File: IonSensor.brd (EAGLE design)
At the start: 50.8 x 22.9 mm, 44 parts, among them IC1 QUAD_OPAMPD, IC2 QUAD_OPAMPD, IC3 QUAD_OPAMPD, X1 B5B-XH-2

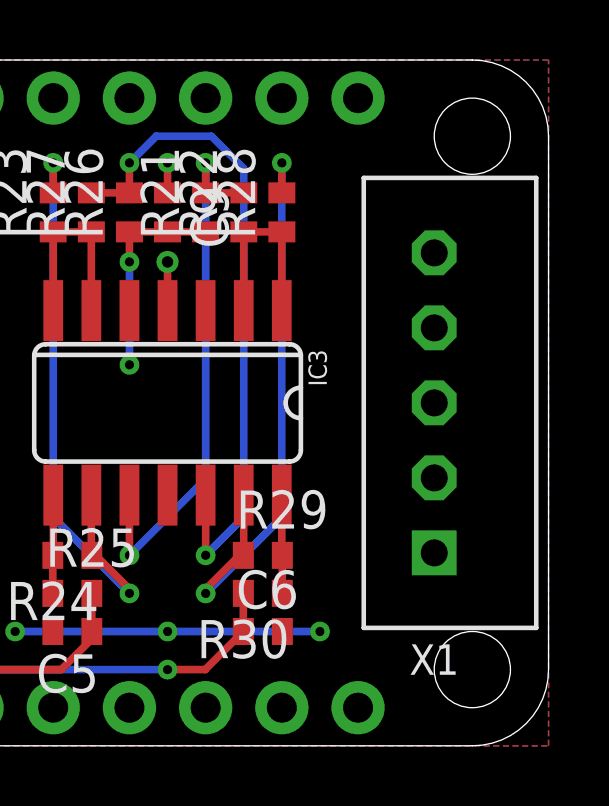
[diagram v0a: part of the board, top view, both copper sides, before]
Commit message: Revert "Added JST XH Connector"
This reverts commit 28e9dc296f10d82968848f6f33b36970200c6171.
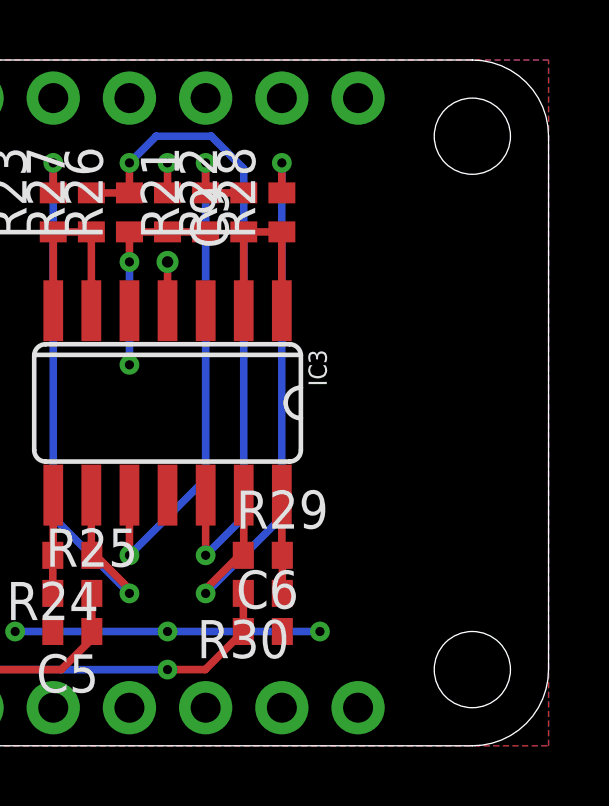
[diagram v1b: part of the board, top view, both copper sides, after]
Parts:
- removed X1: B5B-XH-2, con-JST XH:B5B-XH-A
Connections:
- net CH0: no longer X1.4
- net CH1: no longer X1.3
- net CH2: no longer X1.2
- net GND: no longer X1.1
- net REF: no longer X1.5
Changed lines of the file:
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@@
 <attribute name="VALUE" x="36.068" y="18.669" size="1.27" layer="27" rot="R270"/>
-</element>
-<element name="X1" library="con-JST XH" package="B5B-XH-A" value="B5B-XH-2" x="46.99" y="11.43" smashed="yes" rot="R270">
-<attribute name="NAME" x="46.99" y="3.382" size="1.016" layer="25" rot="R180" align="bottom-center"/>
-<attribute name="VALUE" x="48.26" y="6.43" size="1.016" layer="27" rot="R270" align="bottom-right"/>
 </element>
 </elements>
@@
 <wire x1="24.13" y1="16.129" x2="24.13" y2="12.7" width="0.254" layer="16"/>
 <wire x1="36.83" y1="16.129" x2="36.83" y2="12.7" width="0.254" layer="16"/>
-<contactref element="X1" pad="1"/>
-<wire x1="38.1" y1="8.3566" x2="36.83" y2="12.7" width="0" layer="19" extent="1-1"/>
-<wire x1="38.1" y1="3.81" x2="38.1" y2="8.3566" width="0" layer="19" extent="1-1"/>
-<wire x1="41.925" y1="3.81" x2="43.18" y2="3.81" width="0" layer="19" extent="1-1"/>
-<wire x1="34.275" y1="3.81" x2="33.02" y2="3.81" width="0" layer="19" extent="1-1"/>
-<wire x1="30.48" y1="3.81" x2="33.02" y2="3.81" width="0" layer="19" extent="1-1"/>
-<wire x1="29.225" y1="3.81" x2="30.48" y2="3.81" width="0" layer="19" extent="1-1"/>
-<wire x1="21.575" y1="3.81" x2="20.32" y2="3.81" width="0" layer="19" extent="1-1"/>
-<wire x1="17.78" y1="3.81" x2="20.32" y2="3.81" width="0" layer="19" extent="1-1"/>
-<wire x1="16.525" y1="3.81" x2="17.78" y2="3.81" width="0" layer="19" extent="1-1"/>
-<wire x1="8.875" y1="3.81" x2="7.62" y2="3.81" width="0" layer="19" extent="1-1"/>
-<wire x1="25.4" y1="8.3566" x2="25.4" y2="3.81" width="0" layer="19" extent="1-1"/>
-<wire x1="24.13" y1="12.7" x2="25.4" y2="8.3566" width="0" layer="19" extent="1-1"/>
-<wire x1="12.7" y1="8.3566" x2="12.7" y2="3.81" width="0" layer="19" extent="1-1"/>
-<wire x1="11.43" y1="12.7" x2="12.7" y2="8.3566" width="0" layer="19" extent="1-1"/>
-<wire x1="46.99" y1="6.43" x2="7.62" y2="3.81" width="0" layer="19" extent="1-1"/>
 </signal>
 <signal name="+3V3">
@@
 <signal name="CH0">
 <contactref element="IC1" pad="3"/>
-<contactref element="X1" pad="4"/>
-<wire x1="46.99" y1="13.93" x2="13.97" y2="14.5034" width="0" layer="19" extent="1-1"/>
 </signal>
 <signal name="CH1">
 <contactref element="IC2" pad="3"/>
-<contactref element="X1" pad="3"/>
-<wire x1="46.99" y1="11.43" x2="26.67" y2="14.5034" width="0" layer="19" extent="1-1"/>
 </signal>
 <signal name="CH2">
 <contactref element="IC3" pad="3"/>
-<contactref element="X1" pad="2"/>
-<wire x1="46.99" y1="8.93" x2="39.37" y2="14.5034" width="0" layer="19" extent="1-1"/>
 </signal>
 <signal name="REF">
@@
 <contactref element="IC2" pad="5"/>
 <contactref element="IC3" pad="5"/>
-<contactref element="X1" pad="5"/>
 <wire x1="24.13" y1="14.5034" x2="36.83" y2="14.5034" width="0" layer="19" extent="1-1"/>
 <wire x1="11.43" y1="14.5034" x2="24.13" y2="14.5034" width="0" layer="19" extent="1-1"/>
-<wire x1="46.99" y1="16.43" x2="11.43" y2="14.5034" width="0" layer="19" extent="1-1"/>
 </signal>
 <signal name="C1+">
